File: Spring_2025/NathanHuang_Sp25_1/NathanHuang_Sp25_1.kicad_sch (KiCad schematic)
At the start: 19 parts, among them J1 Barrel_Jack, M1 Motor_Servo, M2 Motor_Servo, M3 Motor_Servo, M4 Motor_Servo, M5 Motor_Servo, M6 Motor_Servo, M7 Stepper_Motor_bipolar, SW1 SW_Push, SW2 SW_Push, U2 LM2596_BUCK_CONVERTER, U3 ESP32-WROOM-32

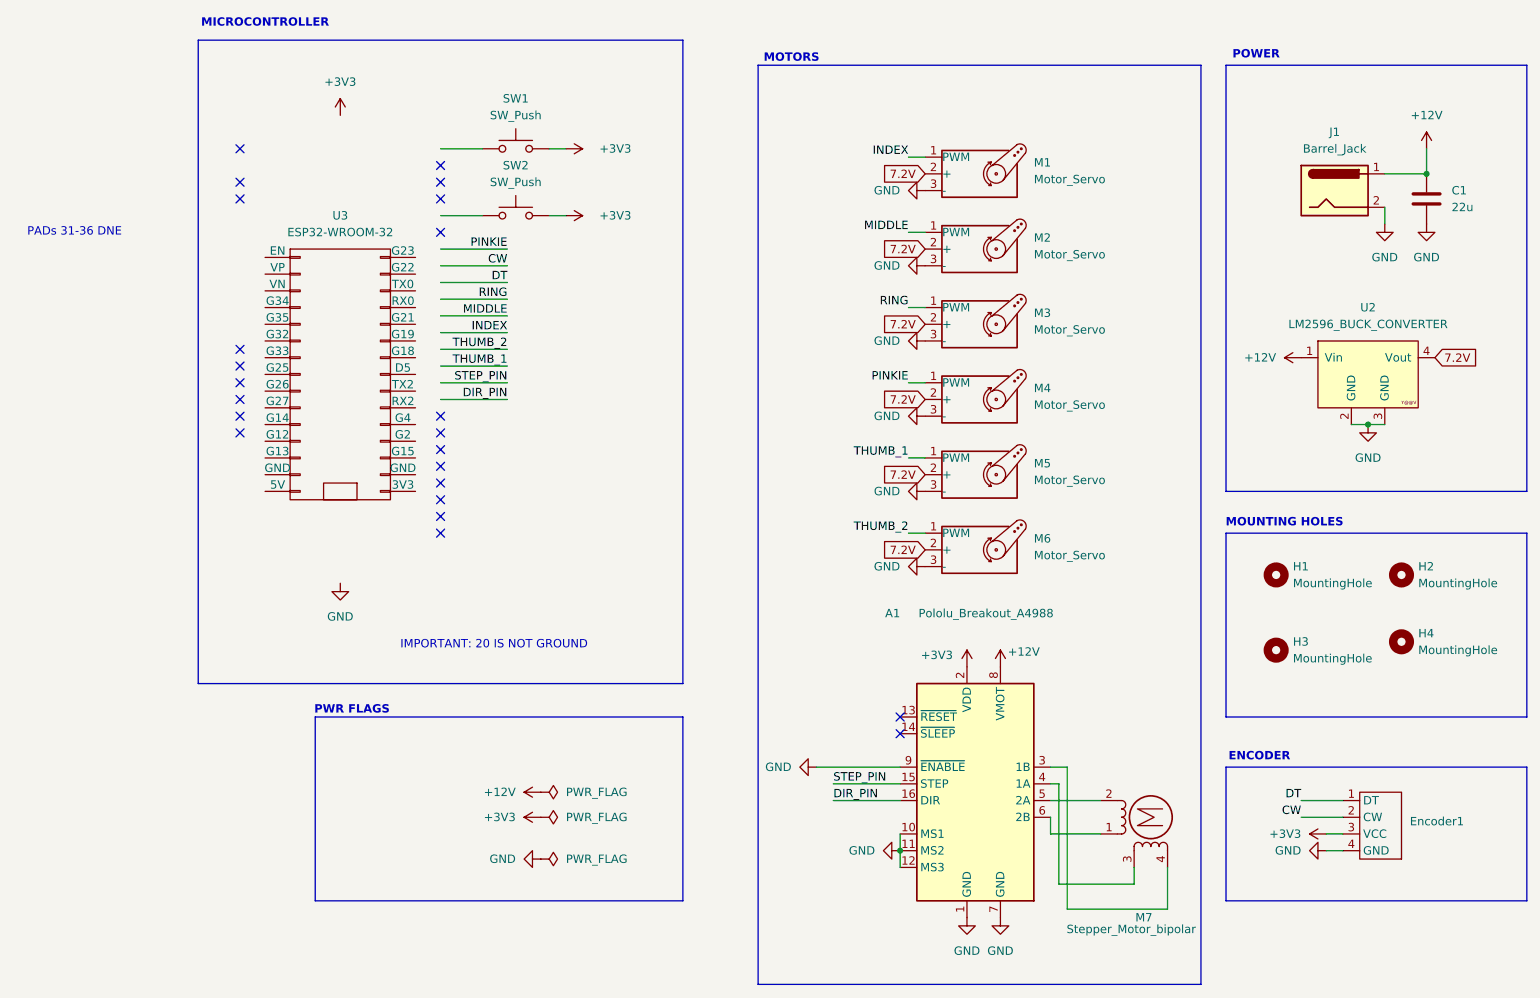
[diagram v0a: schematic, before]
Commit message: Overwrite Changes
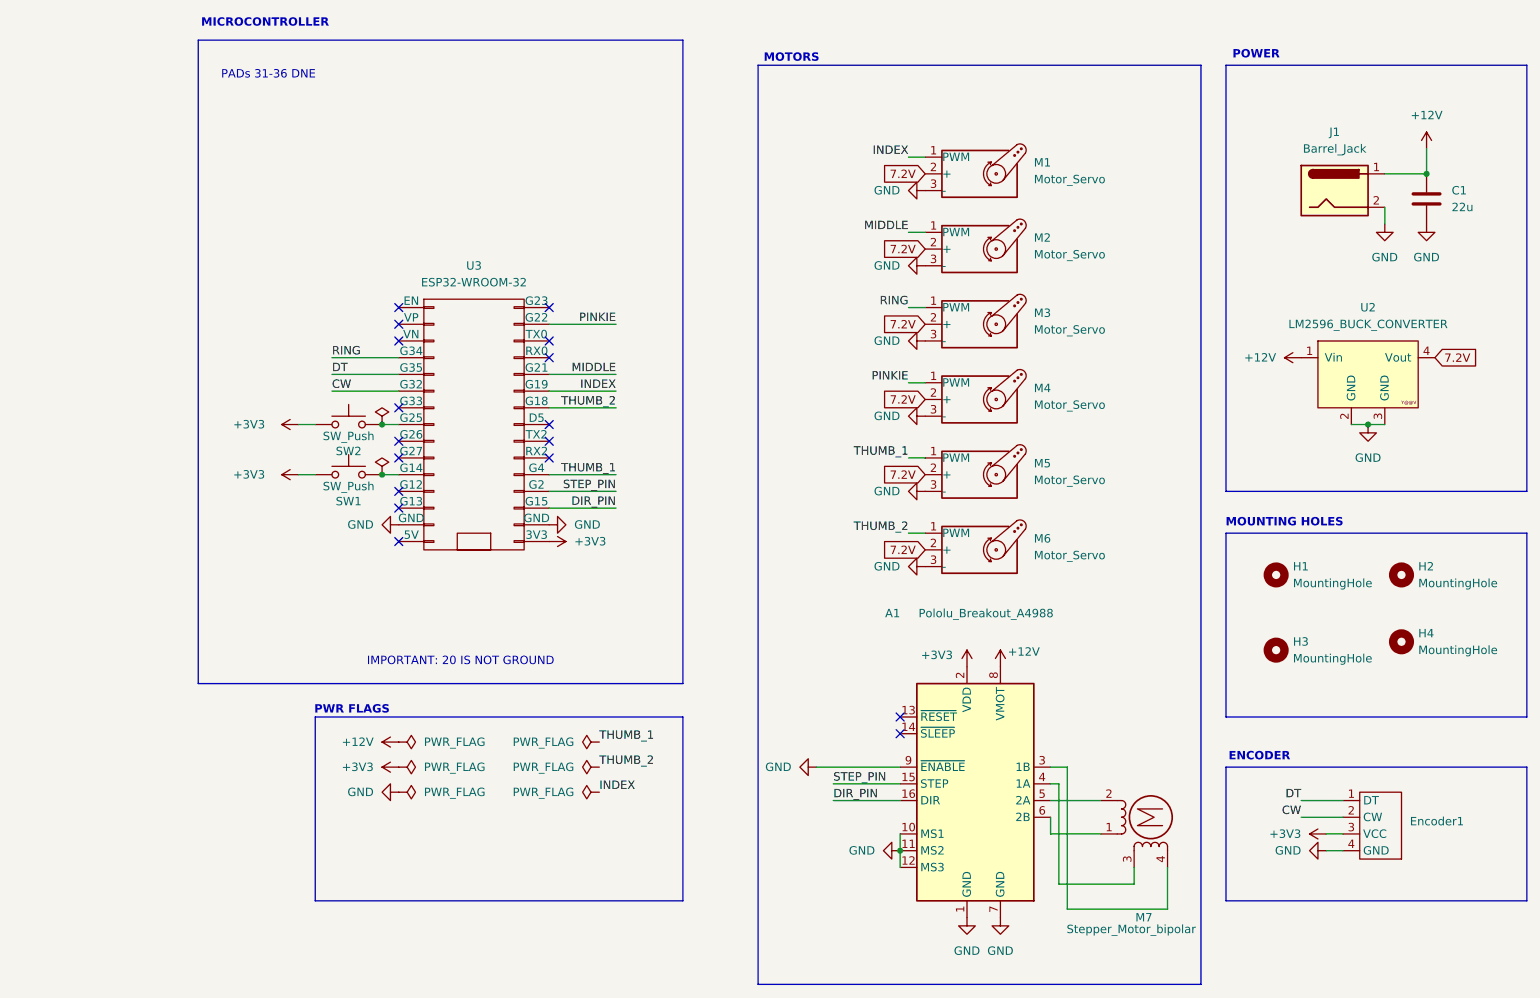
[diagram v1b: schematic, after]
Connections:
- net +3V3: now also U3.30 (3V3)
- net CW: now also U3.6 (G32)
- net DIR_PIN: now also U3.28 (G15)
- net DT: now also U3.5 (G35)
- net GND: now also U3.14 (GND), U3.29 (GND)
- net INDEX: now also U3.21 (G19)
- net MIDDLE: now also U3.20 (G21)
- net PINKIE: now also U3.17 (G22)
- net RING: now also U3.4 (G34)
- net STEP_PIN: now also U3.27 (G2)
- net THUMB_1: now also U3.26 (G4)
- net THUMB_2: now also U3.22 (G18)
- net at SW1.1: now also U3.11 (G14)
- net at SW2.1: now also U3.8 (G25)
- no-connect marks 23 -> 17
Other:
- moved on the sheet: SW1, SW2, U3
